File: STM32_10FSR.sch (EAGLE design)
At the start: 17 parts, among them IC3 7805TV, IC4 UA741P, J1 61302011121, J2 61302011121, U2 HCF4051BEY, X4 057-006-1, X5 057-010-1

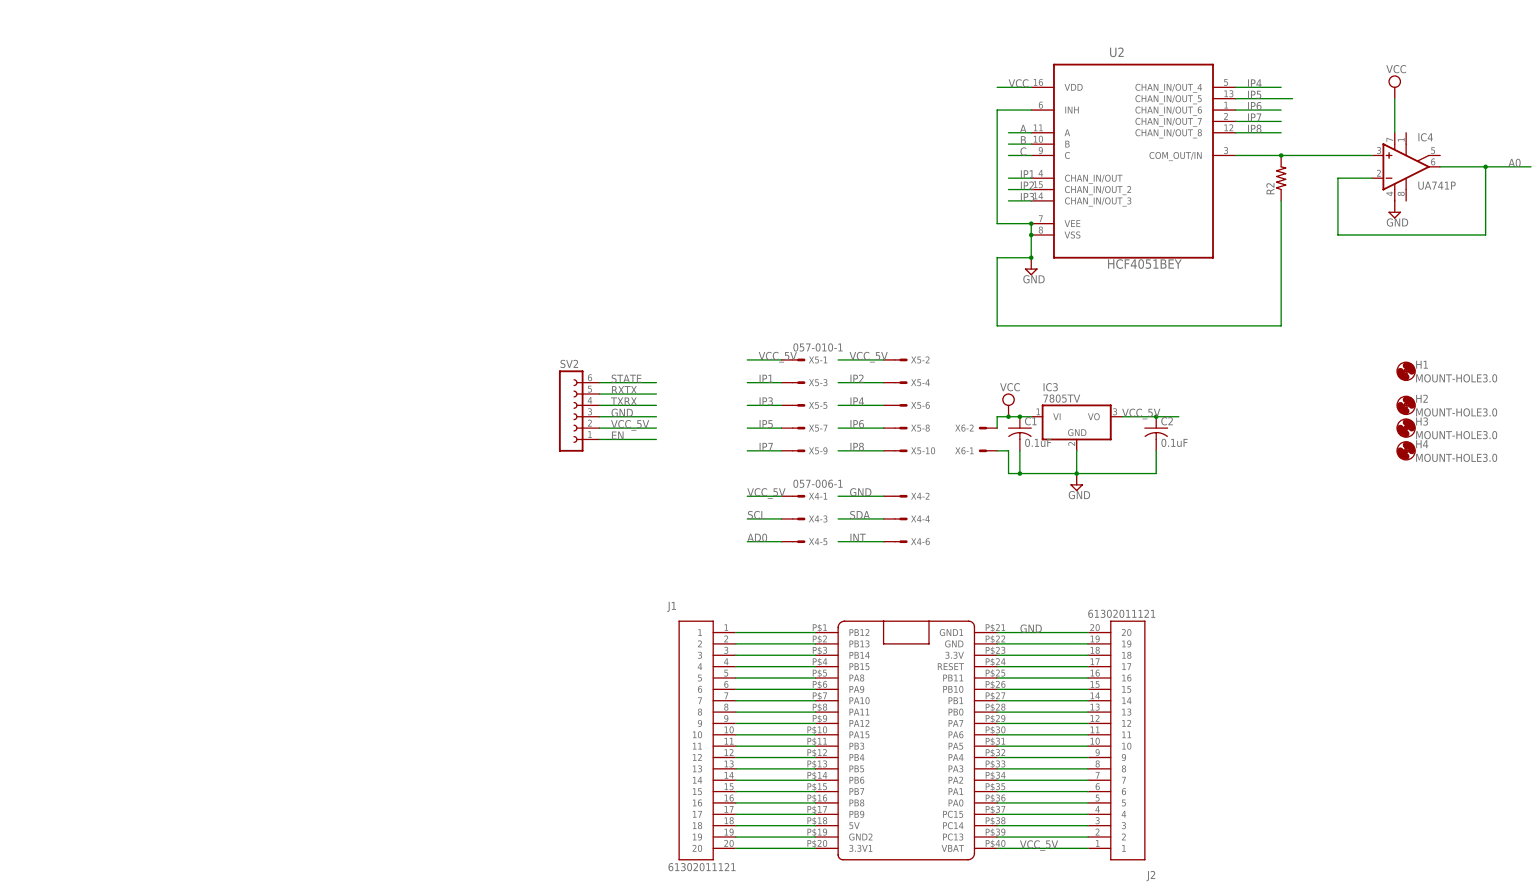
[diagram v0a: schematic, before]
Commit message: 04032020
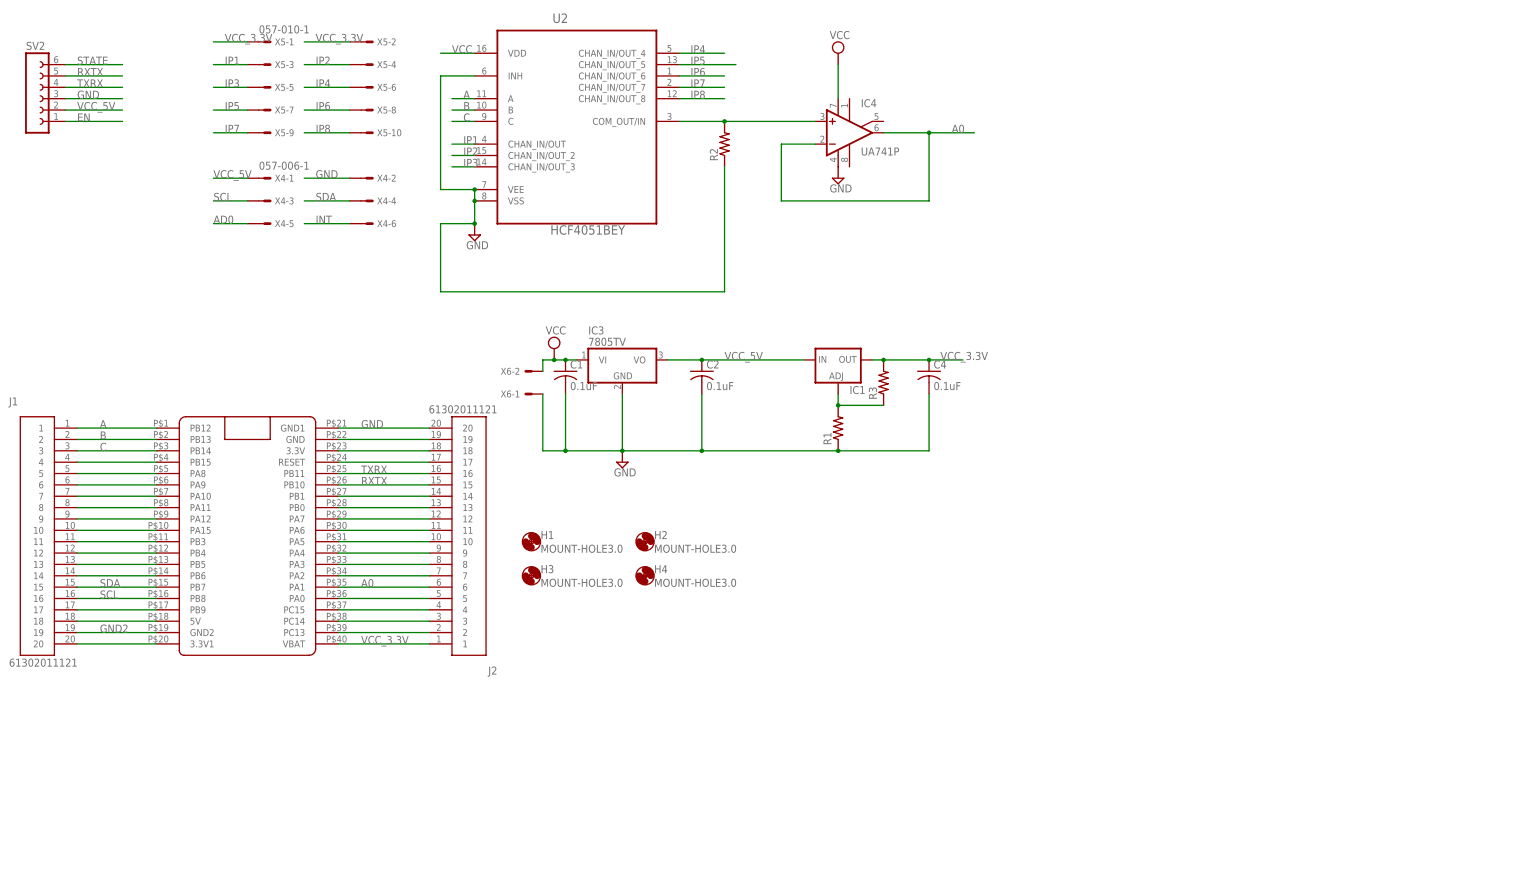
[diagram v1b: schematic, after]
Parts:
- added C4: 0.1uF, rcl:C-US025-024X044
- added IC1: (no value), v-reg:LM317TS
- added R1, R3: (no value), rcl:R-US_0204/7
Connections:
- net N$19 renamed GND2
- removed net N$1 (its old number): J1.1, U$1.PB12
- removed net N$15: J1.15, U$1.PB7
- removed net N$16: J1.16, U$1.PB8
- removed net N$2 (its old number): J1.2, U$1.PB13
- removed net N$26: J2.6, U$1.PA1
- removed net N$3 (its old number): J1.3, U$1.PB14
- removed net N$35: J2.15, U$1.PB10
- removed net N$36: J2.16, U$1.PB11
- new net N$21: IC1.ADJ, R1.2, R3.1
- new net VCC_3.3V: C4.1, IC1.OUT, J2.1, R3.2, U$1.VBAT, X5-1.S, X5-2.S
- net A: now also J1.1, U$1.PB12
- net A0: now also J2.6, U$1.PA1
- net B: now also J1.2, U$1.PB13
- net C: now also J1.3, U$1.PB14
- net GND: now also C4.2, R1.1
- net RXTX: now also J2.15, U$1.PB10
- net SCL: now also J1.16, U$1.PB8
- net SDA: now also J1.15, U$1.PB7
- net TXRX: now also J2.16, U$1.PB11
- net VCC_5V: now also IC1.IN; no longer J2.1, U$1.VBAT, X5-1.S, X5-2.S
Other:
- moved on the sheet: C1, C2, H1, H2, H3, H4, IC3, IC4, J1, J2, R2, SV2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
